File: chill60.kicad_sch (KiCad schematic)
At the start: 7 parts, among them J1 Molex_Pico-EZmate_78171-0004_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, SW1 RST, SW2 BOOT, U1 STM32F072CBTx, U2 XC6206PxxxMR

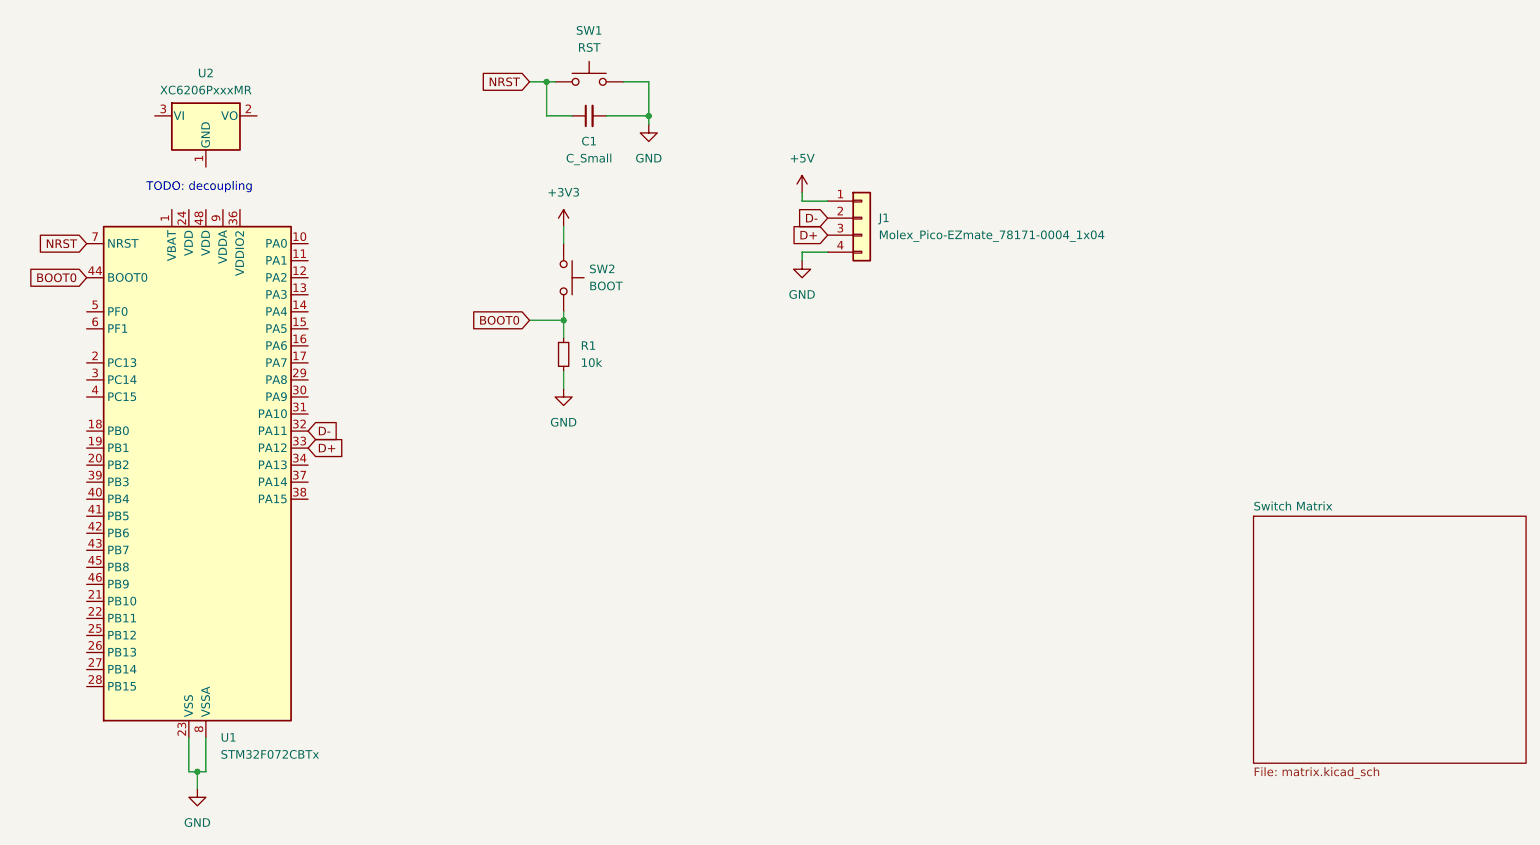
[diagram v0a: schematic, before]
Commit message: initial complete schematic
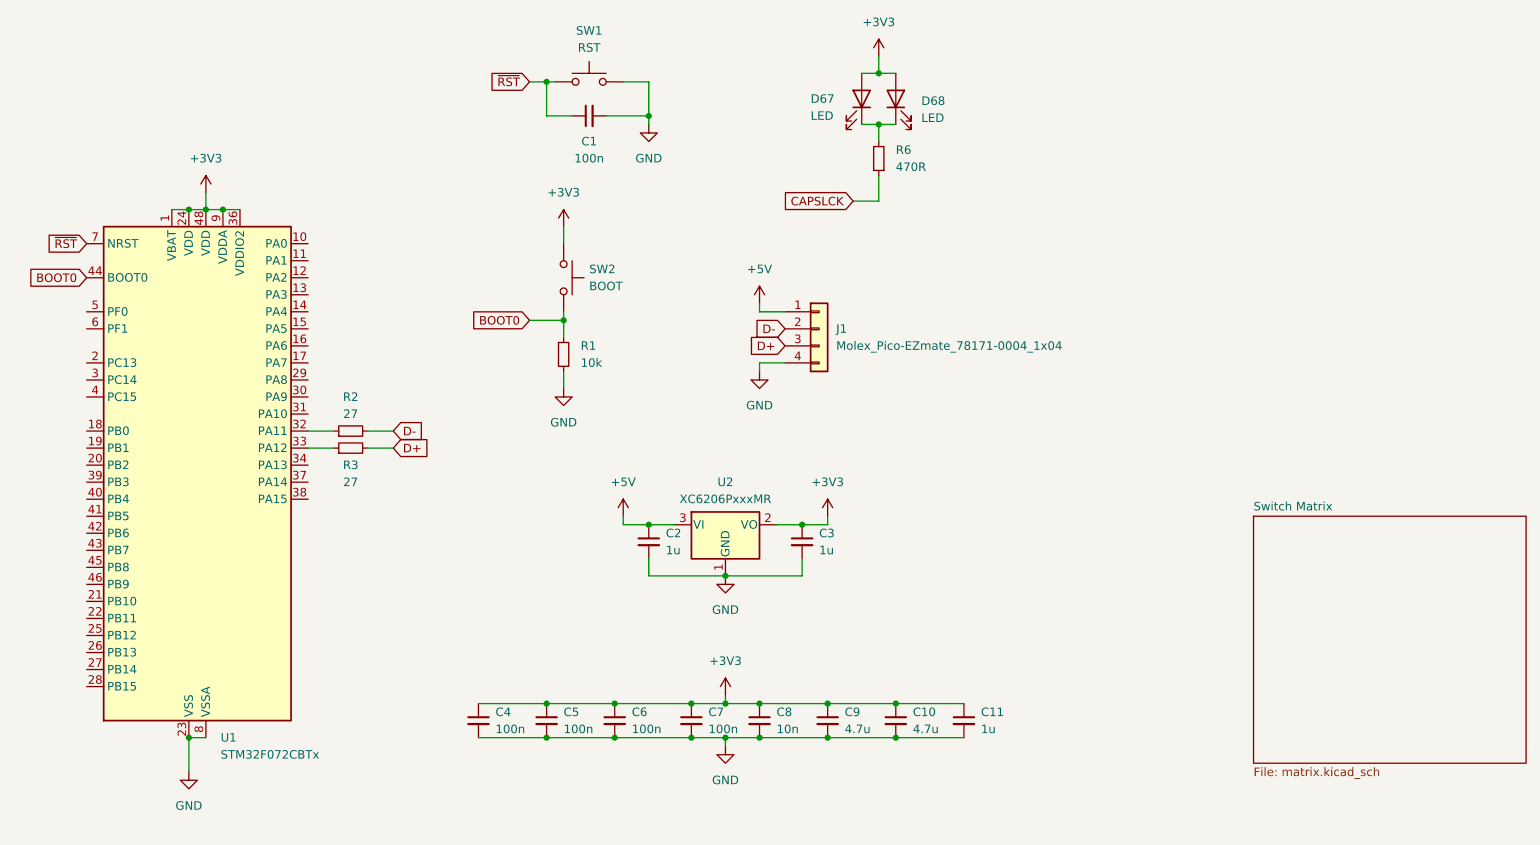
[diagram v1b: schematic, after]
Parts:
- added C10, C9: 4.7u, symbol Device:C_Small
- added C11, C2, C3: 1u, symbol Device:C_Small
- added C4, C5, C6, C7: 100n, symbol Device:C_Small
- added C8: 10n, symbol Device:C_Small
- added D67: LED, marbastlib-mx:LED_MX_3mm, symbol Device:LED
- added D68: LED, marbastlib-mx:LED_MX_3mm-FLIPPED, symbol Device:LED
- added R2, R3: 27, symbol Device:R_Small
- added R6: 470R, Resistor_SMD:R_0402_1005Metric, symbol Device:R_Small
- C1: value C_Small -> 100n
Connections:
- net +3V3: now also U1.1 (VBAT), U1.24 (VDD), U1.36 (VDDIO2), U1.48 (VDD), U1.9 (VDDA), U2.2 (VO), C10.1, C11.1, C3.1, C4.1, C5.1, C6.1, C7.1, C8.1, C9.1, D67.2 (A), D68.2 (A)
- net +5V: now also U2.3 (VI), C2.1
- net D+: now also R3.2; no longer U1.33 (PA12)
- net D-: now also R2.2; no longer U1.32 (PA11)
- net GND: now also U2.1 (GND), C10.2, C11.2, C2.2, C3.2, C4.2, C5.2, C6.2, C7.2, C8.2, C9.2
- net NRST renamed ~{RST}
- new net: R2.1, U1.32 (PA11)
- new net: D67.1 (K), D68.1 (K), R6.2
- new net: R3.1, U1.33 (PA12)
- new net CAPSLCK: R6.1
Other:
- note removed: "TODO: decoupling"
- moved on the sheet: J1, U2
